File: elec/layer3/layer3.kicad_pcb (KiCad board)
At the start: 2 copper layers, 125 x 125 mm, 55 parts, among them J10 Conn_01x05, J4 Conn_01x05, J8 XT30PW-M, J9 XT30PW-M, SW1 SW_SPDT_312, SW2 SW_SPDT_312, SW3 SW_SPDT_312, SW4 SW_SPDT_312, U1 CD74HC4067SM, U2 CD74HC4067SM, U4 4754, U5 113991054

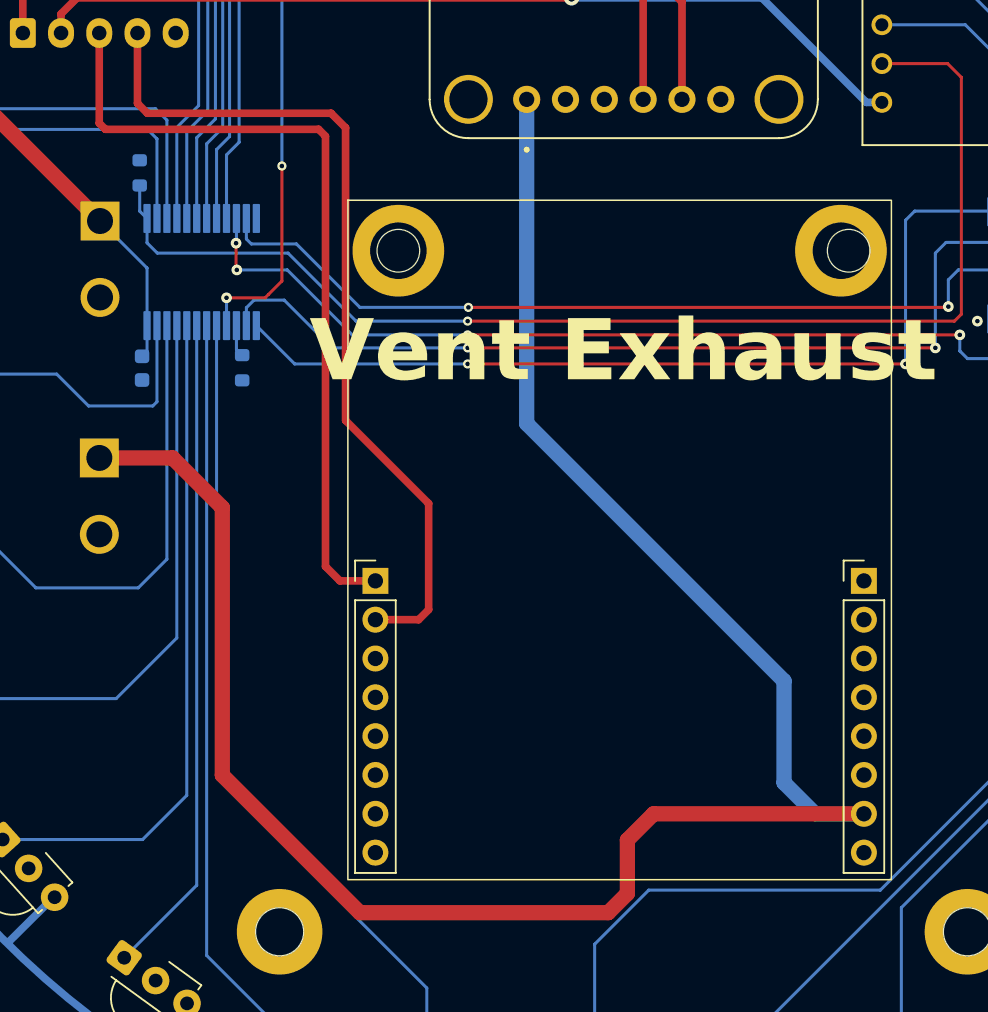
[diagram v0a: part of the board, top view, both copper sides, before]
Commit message: prod: l2, l3
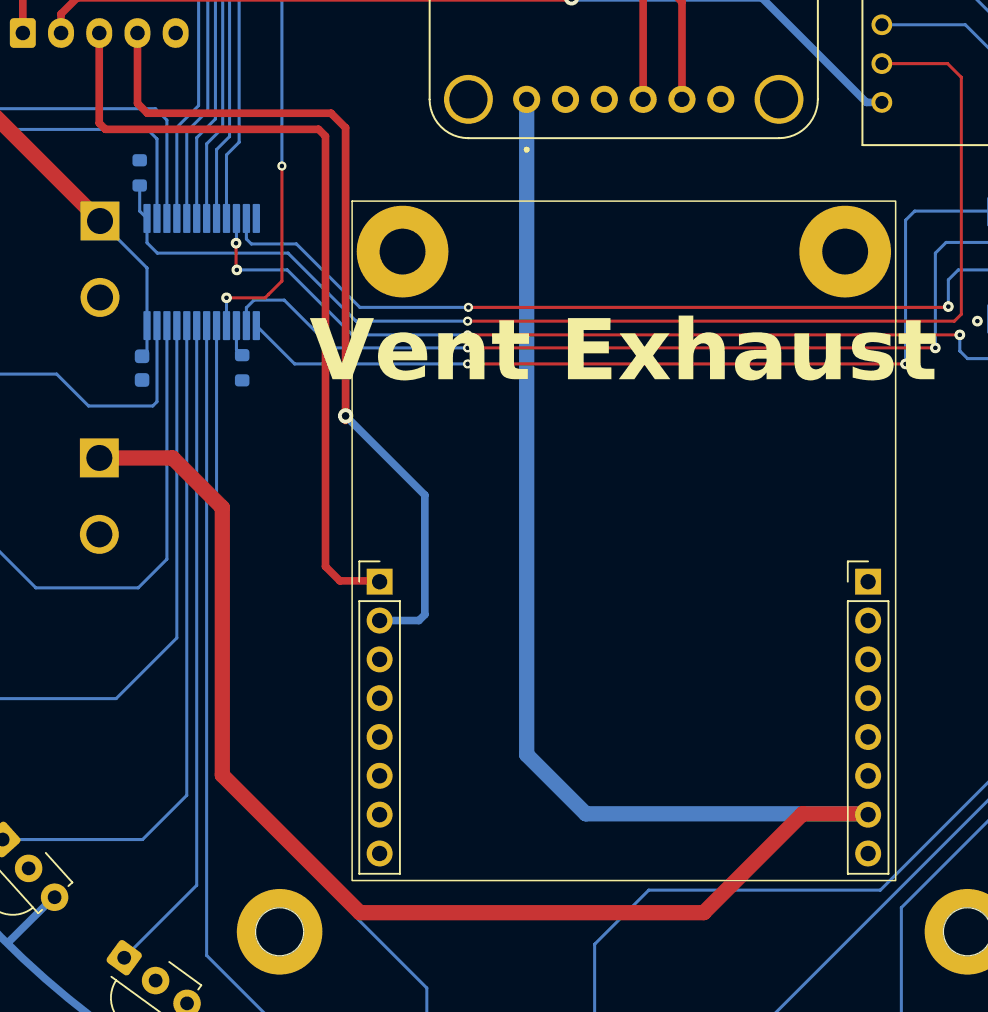
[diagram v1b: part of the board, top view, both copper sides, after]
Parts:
- moved U6 28.7 mm to (146.6, 109.4)
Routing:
- net +5V: track 135.1 -> 142.3 mm
- net /TX (CAM): track 56.4 -> 56.6 mm, vias 0 -> 1
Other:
- outline, holes or cut-outs redrawn
